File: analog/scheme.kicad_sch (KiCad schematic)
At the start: 17 parts, among them U1 LM324N

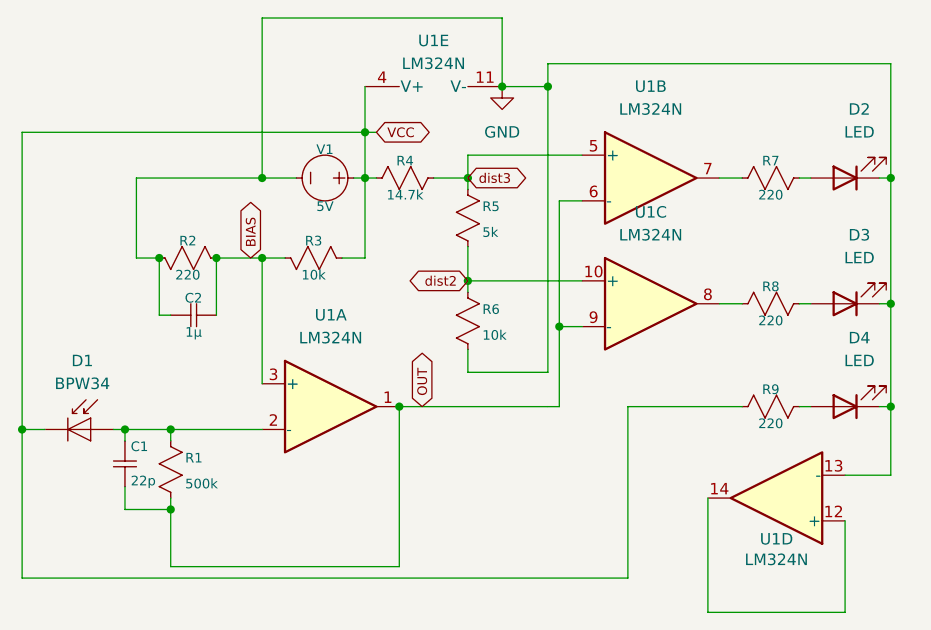
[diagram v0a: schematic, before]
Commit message: Add files via upload
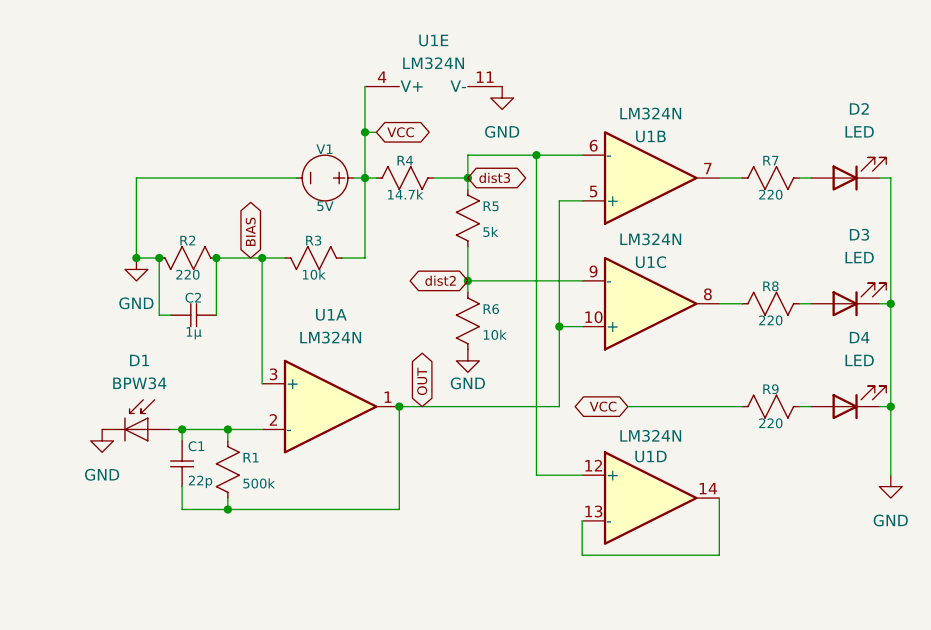
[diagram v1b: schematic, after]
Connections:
- net GND: now also D1.1 (K); no longer U1.13 (-)
- net OUT: now also U1.10 (+), U1.5 (+); no longer U1.6 (-), U1.9 (-)
- net VCC: no longer D1.1 (K)
- net dist2: now also U1.9 (-); no longer U1.10 (+)
- net dist3: now also U1.12 (+), U1.6 (-); no longer U1.5 (+)
- net at U1.14: now also U1.13 (-); no longer U1.12 (+)
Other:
- moved on the sheet: C1, D1, R1, U1D
